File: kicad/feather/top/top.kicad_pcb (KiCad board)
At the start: 2 copper layers, 52 x 25.7 mm, 13 parts, among them J1 Conn_01x12_Socket, J2 Conn_01x16_Socket, J3 Conn_01x03_Socket

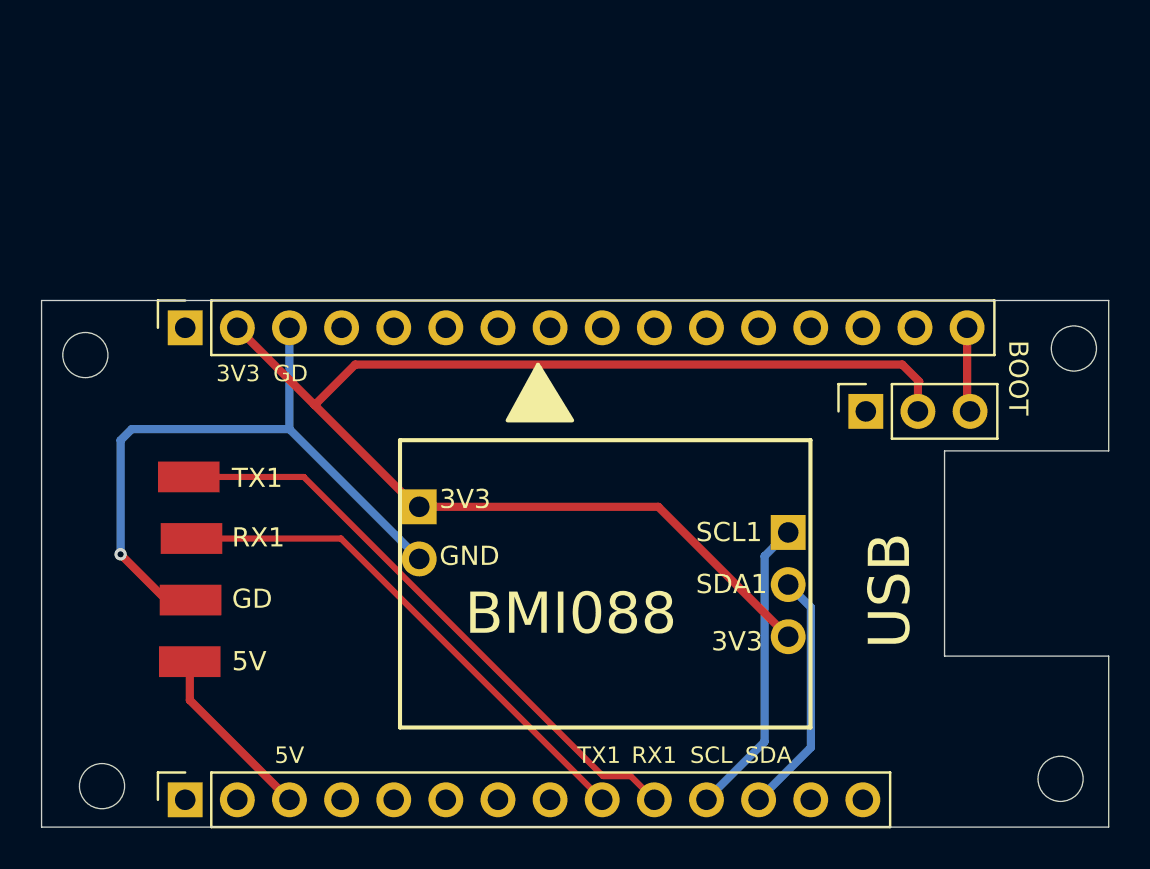
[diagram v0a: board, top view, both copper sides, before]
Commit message: modified:   kicad/feather/top/top.kicad_pro
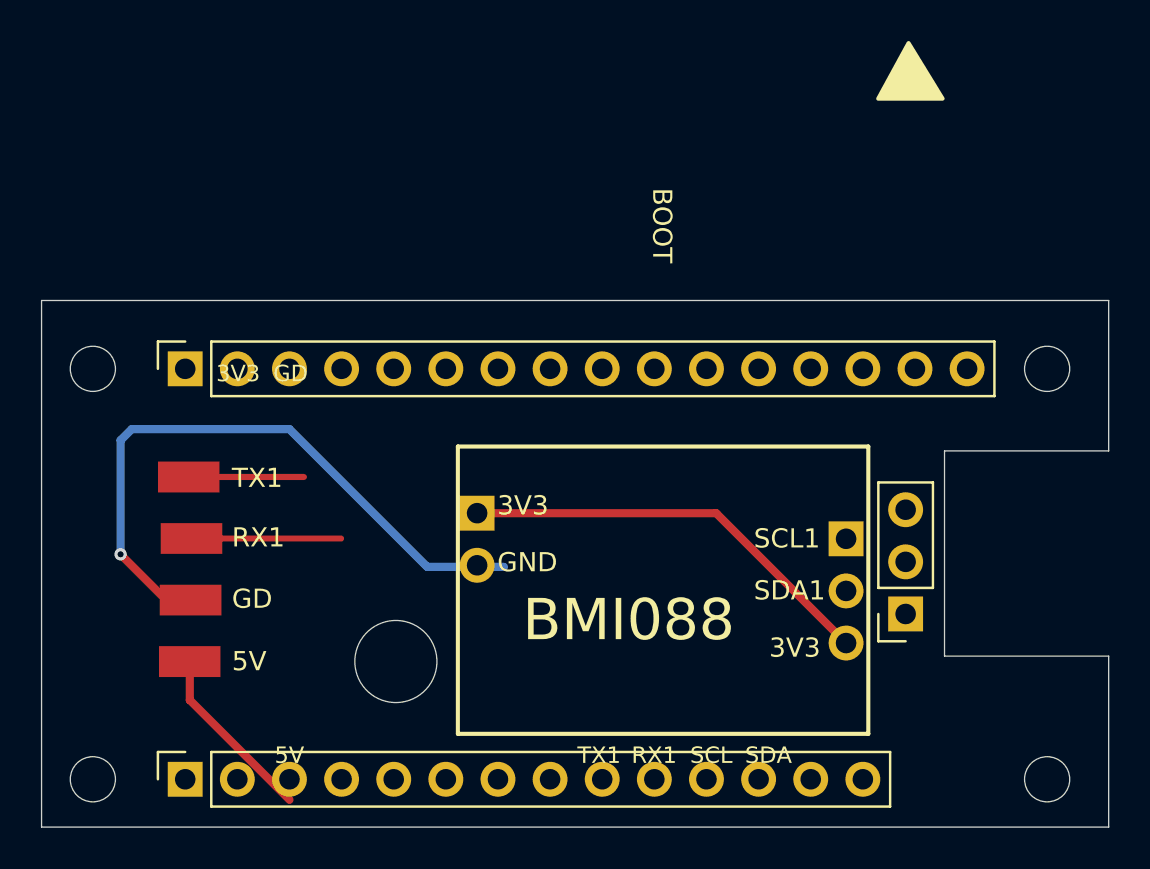
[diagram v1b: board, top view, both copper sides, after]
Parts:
- added POST_5: MountingHole, MountingHole:MountingHole_4mm, F.Cu at (80.3, 116.3)
- moved J3 10.1 mm to (105.1, 113.9), turned to 180 degrees
- moved Motor5 2.84 mm to (101.5, 110.3)
- moved PMW3901_PWR2 2.84 mm to (87.2, 109.0)
- moved J2 2.00 mm to (70.0, 102.0)
- moved POST_2 1.33 mm to (65.1, 100.0)
- moved J1 1.00 mm to (70.0, 122.0)
- moved POST_3 0.65 mm to (112.0, 122.0)
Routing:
- net /3V3: track 65.3 -> 20.9 mm
- net /RX1: track 29.2 -> 7.28 mm
- net /TX1: track 25.3 -> 5.60 mm
- net /SCL: track 14.7 -> 0.00 mm
- net /SDA: track 12.1 -> 0.00 mm
- net /BOOT: track 4.13 -> 0.00 mm
- net /GND: track 32.2 -> 31.6 mm
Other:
- board text removed: "USB"

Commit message: modified:   kicad/feather/top/top.kicad_pro
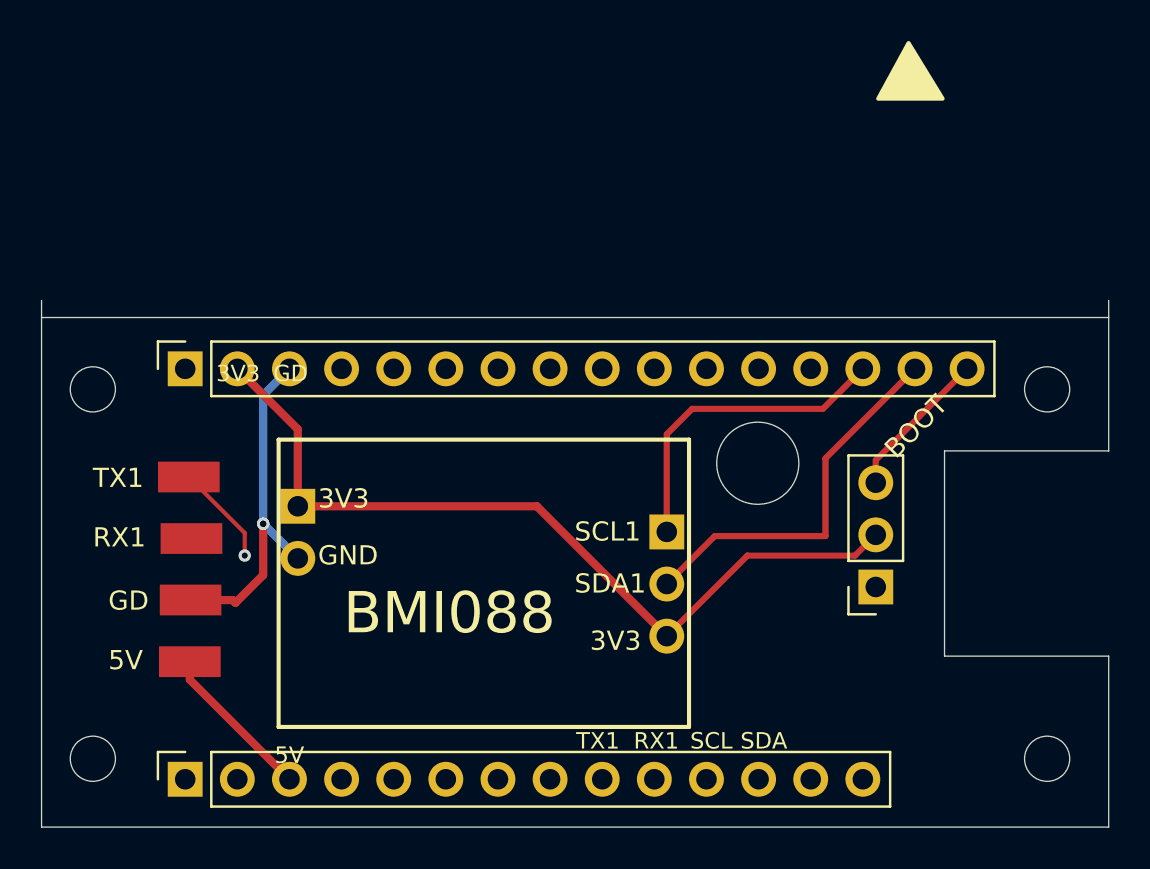
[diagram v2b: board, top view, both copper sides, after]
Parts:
- moved POST_5 20.1 mm to (97.9, 106.6)
- moved Motor5 8.74 mm to (92.7, 109.9)
- moved PMW3901_PWR2 8.74 mm to (78.5, 108.7)
- moved J3 1.96 mm to (103.7, 112.6)
- moved POST_2 1.00 mm to (65.1, 101.0)
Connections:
- J3 pad 2: unconnected-(J3-Pin_2-Pad2) -> /3V3
- J3 pad 3: unconnected-(J3-Pin_3-Pad3) -> /BOOT
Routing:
- net /3V3: track 20.9 -> 41.0 mm
- net /SDA1: track 0.12 -> 18.8 mm
- net /SCL1: track 0.00 -> 15.7 mm
- net /GND: track 31.6 -> 18.3 mm, vias 1 -> 2
- net /BOOT: track 0.00 -> 7.39 mm
- net /RX1: track 7.28 -> 0.00 mm
- net /5V: track 8.74 -> 7.74 mm
- net /TX1: track 5.60 -> 4.96 mm, vias 0 -> 1
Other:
- outline, holes or cut-outs redrawn
